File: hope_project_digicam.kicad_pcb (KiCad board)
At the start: 2 copper layers, 46 parts, among them J1 USB_C_Receptacle_USB2.0_16P, J2 SD_Card_Port, J3 Camera_Pin_Out, J4 Lipo batt in, J5 TFT_Pin_Socket, J6 extra, Q1 NMOS, Q2 PMOS, SW1 SW_Push, SW2 Reset, SW3 Boot, U1 ESP32-S3-WROOM-1, U3 AP2112K-3.3

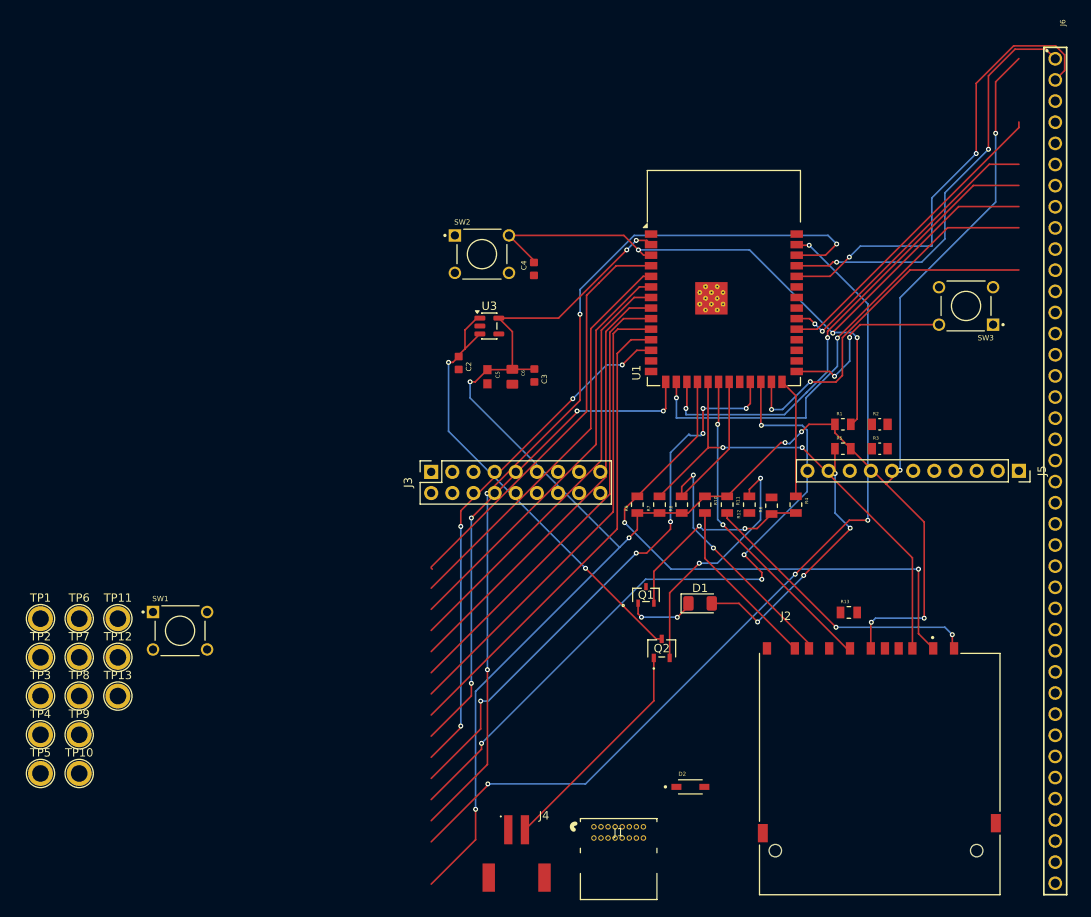
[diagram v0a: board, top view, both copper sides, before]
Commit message: Add files via upload
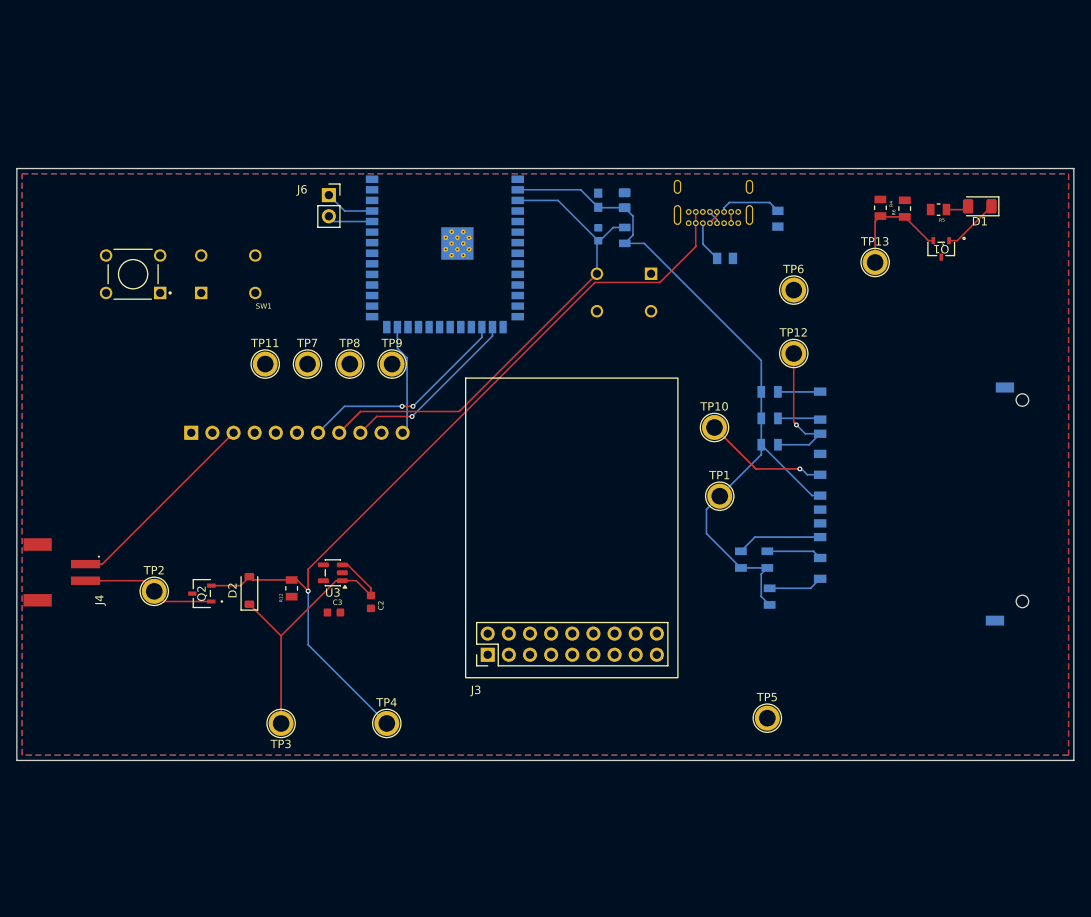
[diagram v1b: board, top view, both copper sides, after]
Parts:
- C4, C5, C6, J2, R1, R10, R11, R13, R2, R3, R7, R8, R9, SW2, SW3, U1: moved to B.Cu
- D2: footprint HOPE DigiCam:Shottky_Diode -> Diode_SMD:D_SOD-123
- J1: footprint HOPE DigiCam:USB_C_Receptacle -> Connector_USB:USB_C_Receptacle_GCT_USB4085; moved to B.Cu
- J3: footprint Connector_PinSocket_2.54mm:PinSocket_2x09_P2.54mm_Vertical -> HOPE DigiCam:Cam Module
- J5: footprint Connector_PinSocket_2.54mm:PinSocket_1x11_P2.54mm_Vertical -> HOPE DigiCam:TFT Module; moved to B.Cu
- J6: footprint HOPE DigiCam:40_Pin_Conn -> Connector_PinSocket_2.54mm:PinSocket_1x02_P2.54mm_Vertical
- SW1: value SW_Push -> Cam Trigger
- moved TP13 104.8 mm to (181.9, 64.0)
- moved TP6 94.5 mm to (172.1, 67.3)
- moved J6 93.4 mm to (116.2, 55.9), turned to 0 degrees
- moved TP12 89.0 mm to (172.1, 74.9)
- moved SW3 88.7 mm to (104.1, 65.4), turned to 0 degrees
- moved TP5 87.6 mm to (168.9, 118.7)
- moved J5 87.1 mm to (112.3, 95.5), turned to 0 degrees
- moved TP10 86.9 mm to (162.6, 83.8)
- moved TP1 82.9 mm to (163.2, 92.1)
- moved J1 73.4 mm to (159.5, 59.3)
- moved J4 60.3 mm to (87.0, 101.2), turned to 90 degrees
- moved D1 58.4 mm to (194.4, 57.2), turned to 180 degrees
- moved TP9 58.3 mm to (123.8, 76.2)
- moved D2 58.0 mm to (106.7, 103.4), turned to 90 degrees
- moved R12 55.9 mm to (111.8, 103.1)
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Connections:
- R2 pad 2: Net-(J1-CC1) -> /CC1
- R3 pad 2: Net-(J1-CC2) -> /CC2
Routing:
- net +3.3V: track 243.3 -> 88.4 mm, vias 11 -> 0
- net /CAM_SDA: track 110.6 -> 0.00 mm, vias 4 -> 0
- net /CAM_SCL: track 106.0 -> 0.00 mm, vias 4 -> 0
- net /CAM_VS: track 84.0 -> 0.00 mm, vias 4 -> 0
- net /VBUS: track 30.1 -> 103.4 mm, vias 2 -> 1
- net /CAM_HS: track 69.0 -> 0.00 mm, vias 6 -> 0
- net /CAM_PC: track 61.9 -> 0.00 mm, vias 4 -> 0
- net /SD_CS: track 68.4 -> 6.68 mm, vias 2 -> 0
- net /CAM_XC: track 60.3 -> 0.00 mm, vias 4 -> 0
- net /CAM_D9: track 57.4 -> 0.00 mm
- net /CAM_D8: track 57.1 -> 0.00 mm
- net /CAM_D7: track 55.4 -> 0.00 mm
- net /CAM_D6: track 53.7 -> 0.00 mm
- net /CAM_D5: track 52.1 -> 0.00 mm
- net /CAM_D4: track 50.5 -> 0.00 mm
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- added copper zone on F.Cu, net +3.3V
- added copper zone on B.Cu, net GND
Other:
- board outline added: 127 x 71.1 mm

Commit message: finished layout pretty much
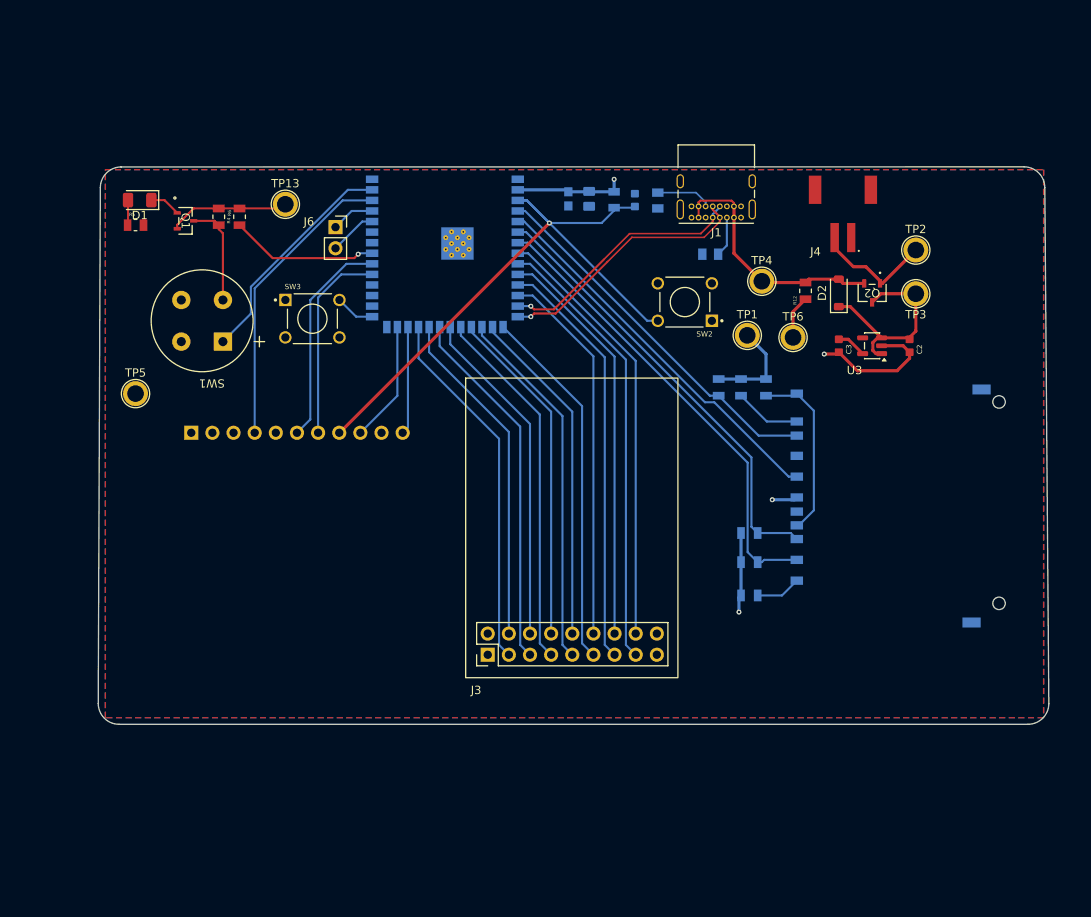
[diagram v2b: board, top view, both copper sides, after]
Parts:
- removed TP10, TP11, TP12, TP7, TP8, TP9: TestPoint, TestPoint:TestPoint_Plated_Hole_D2.0mm
- J1, SW2, SW3: moved to F.Cu
- SW1: footprint HOPE DigiCam:SW2_SW3 -> SWITCH_CAM:D6R_CNK
- moved D1 100.9 mm to (93.5, 56.5)
- moved TP2 100.3 mm to (186.8, 62.5)
- moved J4 99.5 mm to (178.0, 61.0), turned to 0 degrees
- moved R5 96.5 mm to (93.0, 59.5), turned to 0 degrees
- moved TP3 92.1 mm to (186.8, 67.8)
- moved Q1 90.9 mm to (99.0, 59.0), turned to -90 degrees
- moved Q2 88.3 mm to (181.5, 67.7), turned to 180 degrees
- moved TP5 85.3 mm to (93.0, 79.8)
- moved R6 82.4 mm to (103.0, 58.5), turned to -90 degrees
- moved D2 79.3 mm to (177.5, 67.7)
- moved R4 77.0 mm to (105.5, 58.5), turned to 90 degrees
- moved C2 71.7 mm to (186.0, 74.0)
- moved R12 71.3 mm to (173.5, 67.4)
- moved TP13 71.2 mm to (111.0, 57.0)
- moved U3 70.3 mm to (181.5, 74.0)
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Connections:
- U1 pad 10: /CAM_D8 -> /CAM_D4
- U1 pad 11: /CAM_D9 -> /CAM_D5
- U1 pad 12: /CAM_PC -> /CAM_D6
- U1 pad 15: /CAM_XC -> /CAM_D7
- U1 pad 16: /TFT_DC -> /CAM_D8
- U1 pad 17: /TFT_CS -> /CAM_D9
- U1 pad 18: /SD_CS -> /CAM_XC
- U1 pad 19: /SD_MOSI -> /CAM_PC
- U1 pad 20: /SD_SCK -> /CAM_HS
- U1 pad 21: /SD_MISO -> /CAM_VS
- U1 pad 22: /CAM_TRIGGER -> /CAM_SDA
- U1 pad 23: /CAM_HS -> /CAM_SCL
- U1 pad 24: /CAM_VS -> /TFT_LIT
- U1 pad 25: /TFT_LIT -> /TFT_DC
- U1 pad 26: /LED -> unconnected-(U1-IO45-Pad26)
- U1 pad 31: /TFT_SCK -> /TFT_CS
- U1 pad 33: unconnected-(U1-IO40-Pad33) -> /LED
- U1 pad 38: /CAM_SDA -> /TFT_SCK
- U1 pad 39: /CAM_SCL -> /CAM_TRIGGER
- U1 pad 4: /CAM_D2 -> /SD_MISO
- U1 pad 5: /CAM_D3 -> /SD_SCK
- U1 pad 6: /CAM_D4 -> /SD_MOSI
- U1 pad 7: /CAM_D5 -> /SD_CS
- U1 pad 8: /CAM_D6 -> /CAM_D2
- U1 pad 9: /CAM_D7 -> /CAM_D3
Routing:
- net /VBUS: track 103.4 -> 29.8 mm, vias 1 -> 0
- net /CAM_D3: track 0.00 -> 53.7 mm
- net /CAM_D2: track 0.00 -> 52.3 mm
- net /CAM_D5: track 0.00 -> 50.3 mm
- net /SD_CS: track 6.68 -> 55.8 mm
- net /CAM_D4: track 0.00 -> 49.0 mm
- net +3.3V: track 88.4 -> 41.3 mm, vias 0 -> 3
- net /CAM_D6: track 0.00 -> 45.4 mm
- net /CAM_VS: track 0.00 -> 43.9 mm
- net /CAM_PC: track 0.00 -> 43.9 mm
- net /CAM_SCL: track 0.00 -> 43.9 mm
- net /CAM_D9: track 0.00 -> 43.9 mm
- net /CAM_D7: track 0.00 -> 43.9 mm
- net /SD_MOSI: track 10.2 -> 53.7 mm
- net /CAM_HS: track 0.00 -> 40.8 mm
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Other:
- board size 127 x 71.1 mm -> 114.2 x 67 mm
